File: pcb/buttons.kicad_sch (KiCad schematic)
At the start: 92 parts, among them J3 MSP_SBW, SW1 Off, SW10 R_LCD3, SW11 R_LCD4, SW12 LCD_LEFT, SW13 LCD_RIGHT, SW14 Glow, SW15 Device, SW16 Media, SW17 Mute, SW18 Prev, SW19 Vol+, SW2 Activities, SW20 Vol-, SW21 Ch+, SW22 Ch-, SW23 Dpad_Up, SW24 Dpad_Left, SW25 Dpad_Right, SW26 Dpad_Down, SW27 Dpad_OK, SW28 PgUp, SW29 PgDown, SW3 Help, SW30 Menu, SW31 Exit, SW32 Guide, SW33 Info, SW34 Stop, SW35 Replay, SW36 Skip, SW37 Play, SW38 Rec, SW39 Rew, SW4 L_LCD1, SW40 Fwd, SW41 Pause, SW42 KP_1, SW43 KP_2, SW44 KP_3, SW45 KP_4, SW46 KP_5, SW47 KP_6, SW48 KP_7, SW49 KP_8, SW5 L_LCD2, SW50 KP_9, SW51 KP_0, SW52 KP_Clear, SW53 KP_Enter, SW54 SW_RollingBall, SW6 L_LCD3, SW7 L_LCD4, SW8 R_LCD1, SW9 R_LCD2, U1 MSP430G2553IPW28

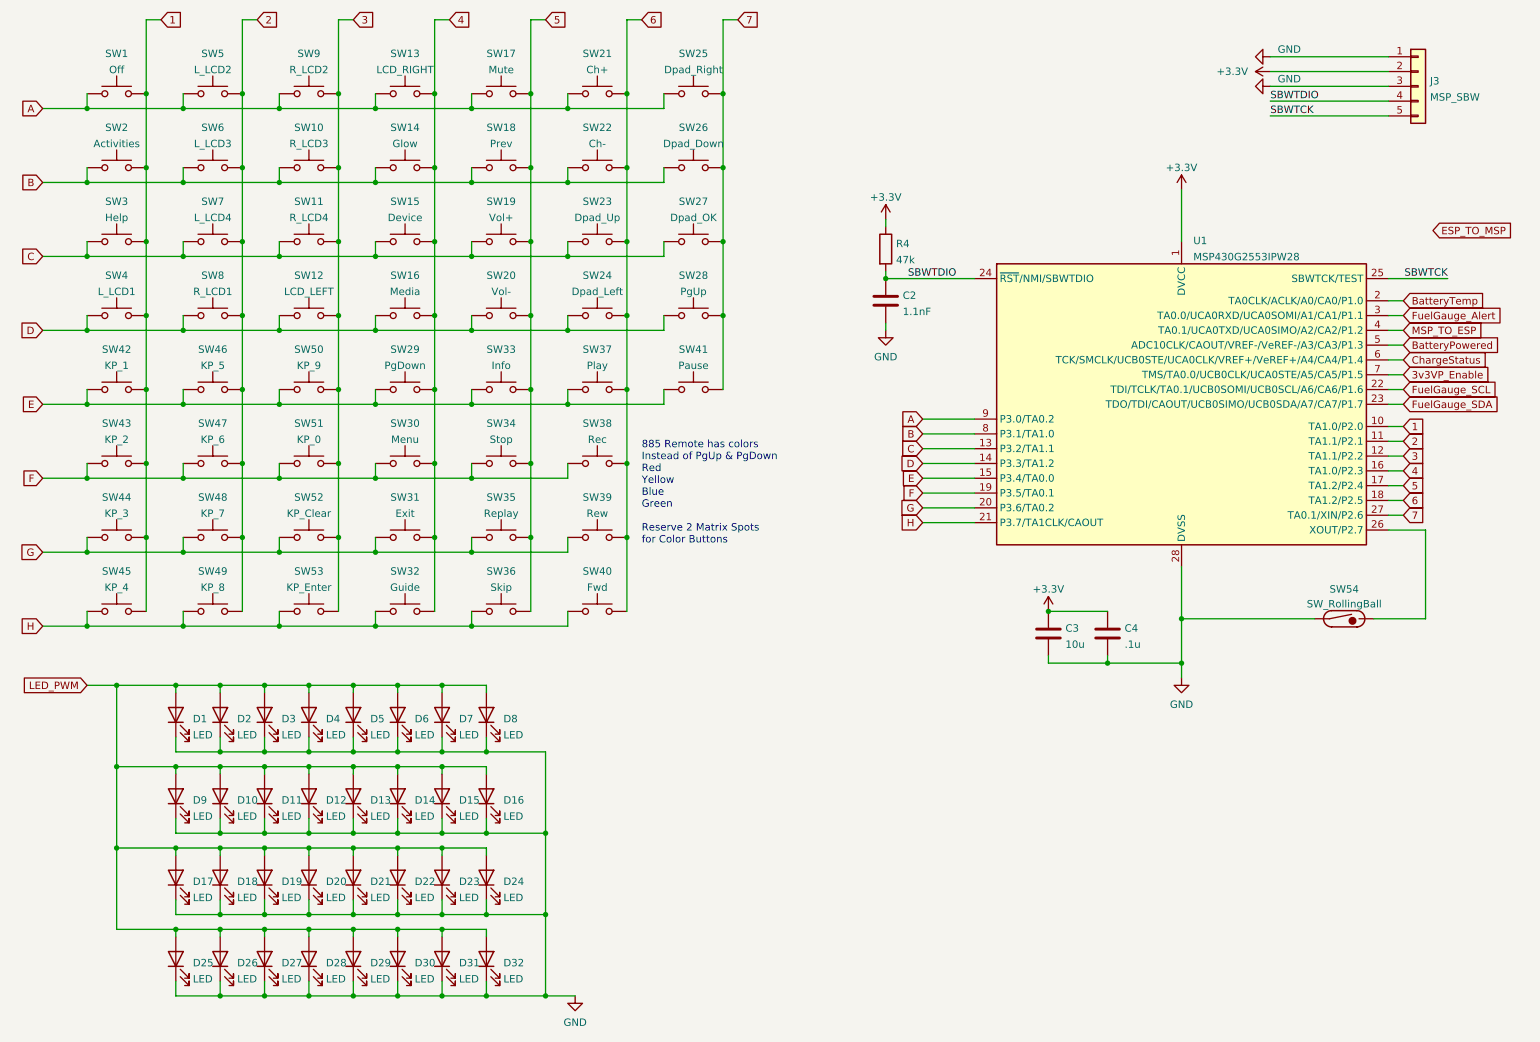
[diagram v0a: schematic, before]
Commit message: more schematic updates
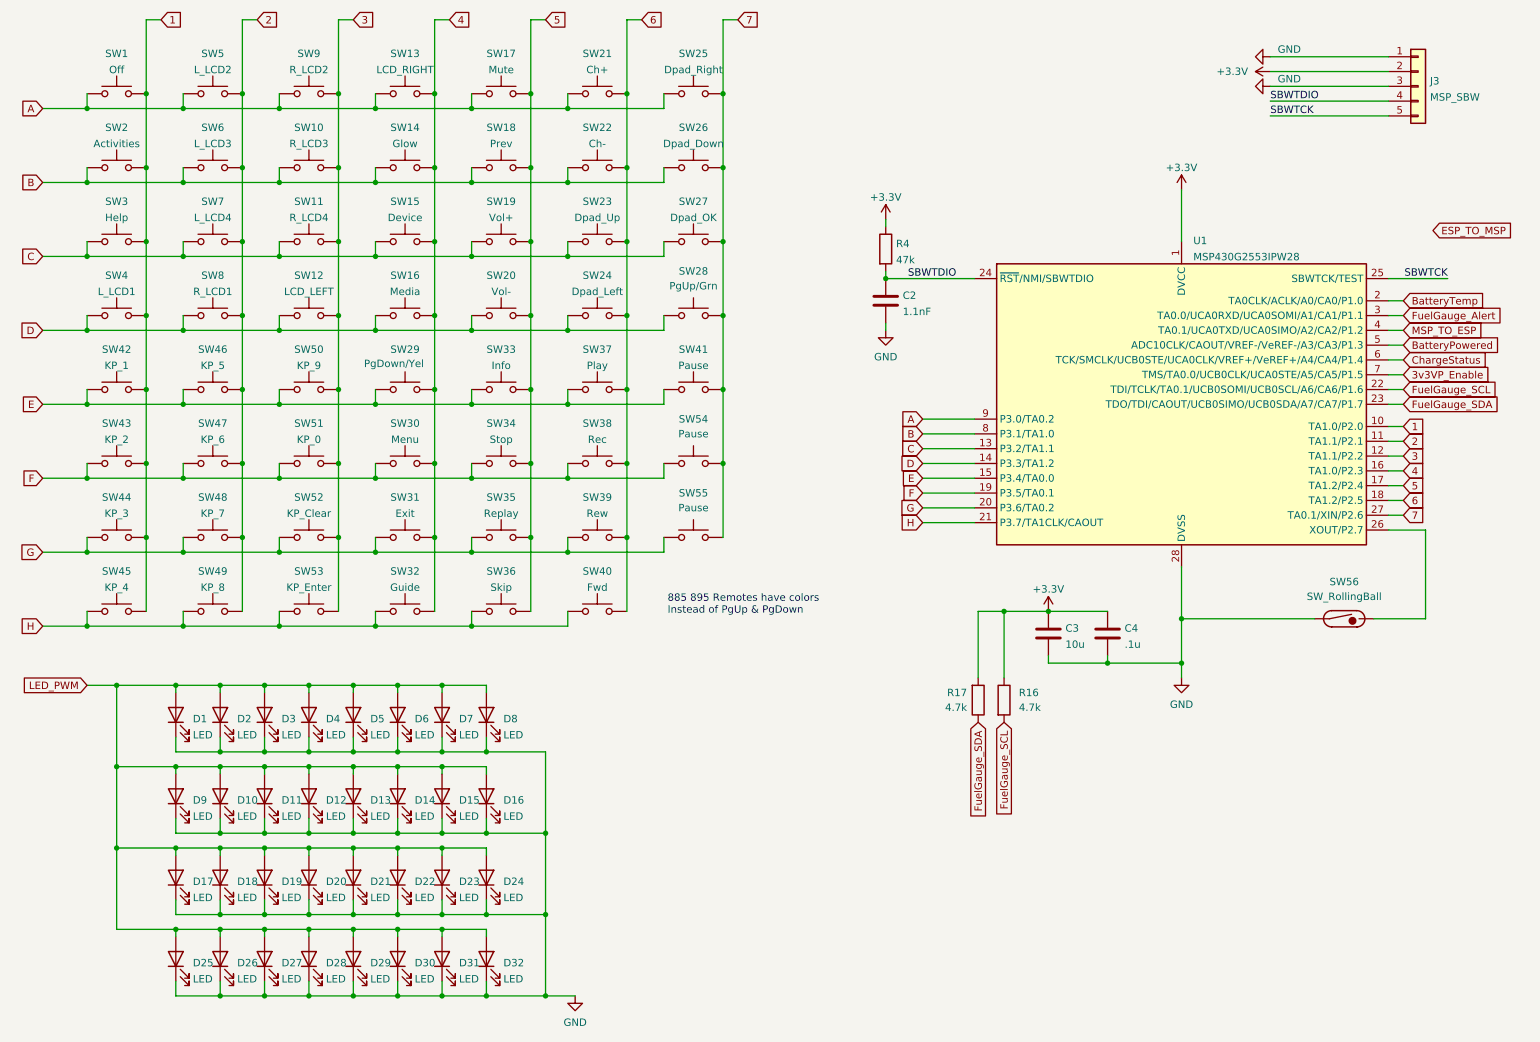
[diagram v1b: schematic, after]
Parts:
- added R16, R17: 4.7k, Resistor_SMD:R_0805_2012Metric, symbol Device:R
- added SW54, SW55: Pause, 880+:4mm Dome, symbol Switch:SW_Push
- SW28: value PgUp -> PgUp/Grn
- SW29: value PgDown -> PgDown/Yel
- renumbered SW54 to SW56
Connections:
- net +3.3V: now also R16.1, R17.2
- net 7: now also SW54.2, SW55.2
- net F: now also SW54.1
- net FuelGauge_SCL: now also R16.2
- net FuelGauge_SDA: now also R17.1
- net G: now also SW55.1
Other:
- note added: "885 895 Remotes have colors Instead of PgUp & PgDown"
- note removed: "885 Remote has colors Instead of PgUp & PgDown Red Yellow Blue Green Reserve 2 Matrix Spots for Color Buttons"
